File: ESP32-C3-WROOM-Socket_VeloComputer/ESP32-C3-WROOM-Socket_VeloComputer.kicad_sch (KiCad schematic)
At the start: 29 parts, among them J1 I2C, J3 Reed_Speed_Socket, J4 USB-C_Receptacle_Data_16P_GCT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, J5 Conn_01x02_Socket, J6 Speed_01x02_Pin, J7 Cadense_01x02_Pin, SW1 SW_Push_SMD_6x3.5, SW2 ENABLE, SW3 SW_Reed_Speed, SW4 SW_Reed_Cadence, U1 ESP32-C3-WROOM-02-N4, U2 AMS1117-3V3, U3 74LS14

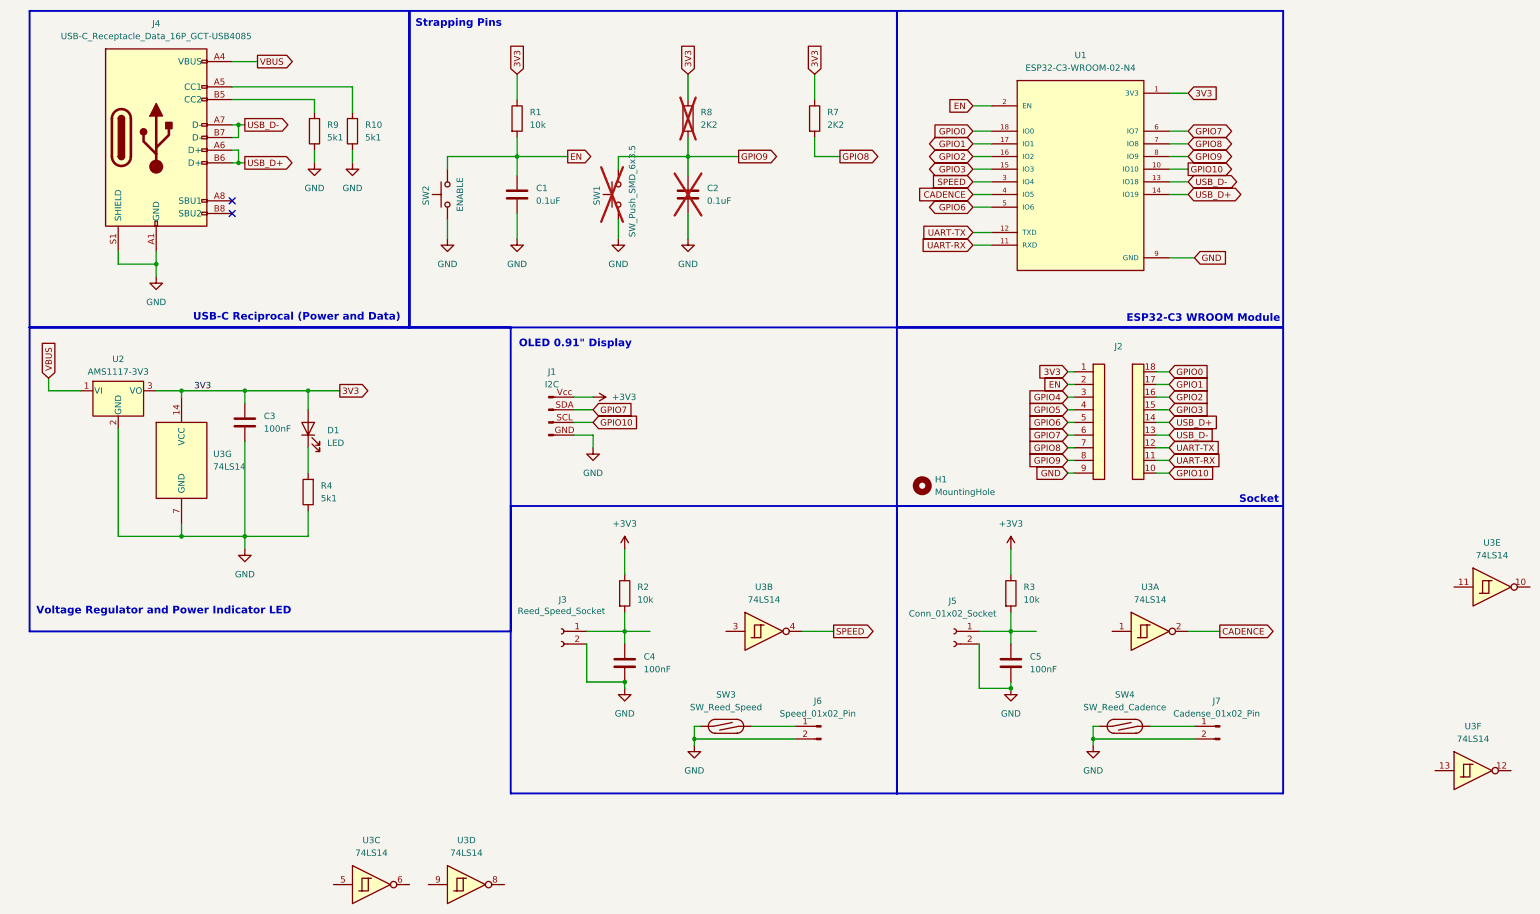
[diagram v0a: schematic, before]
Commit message: velocomputer
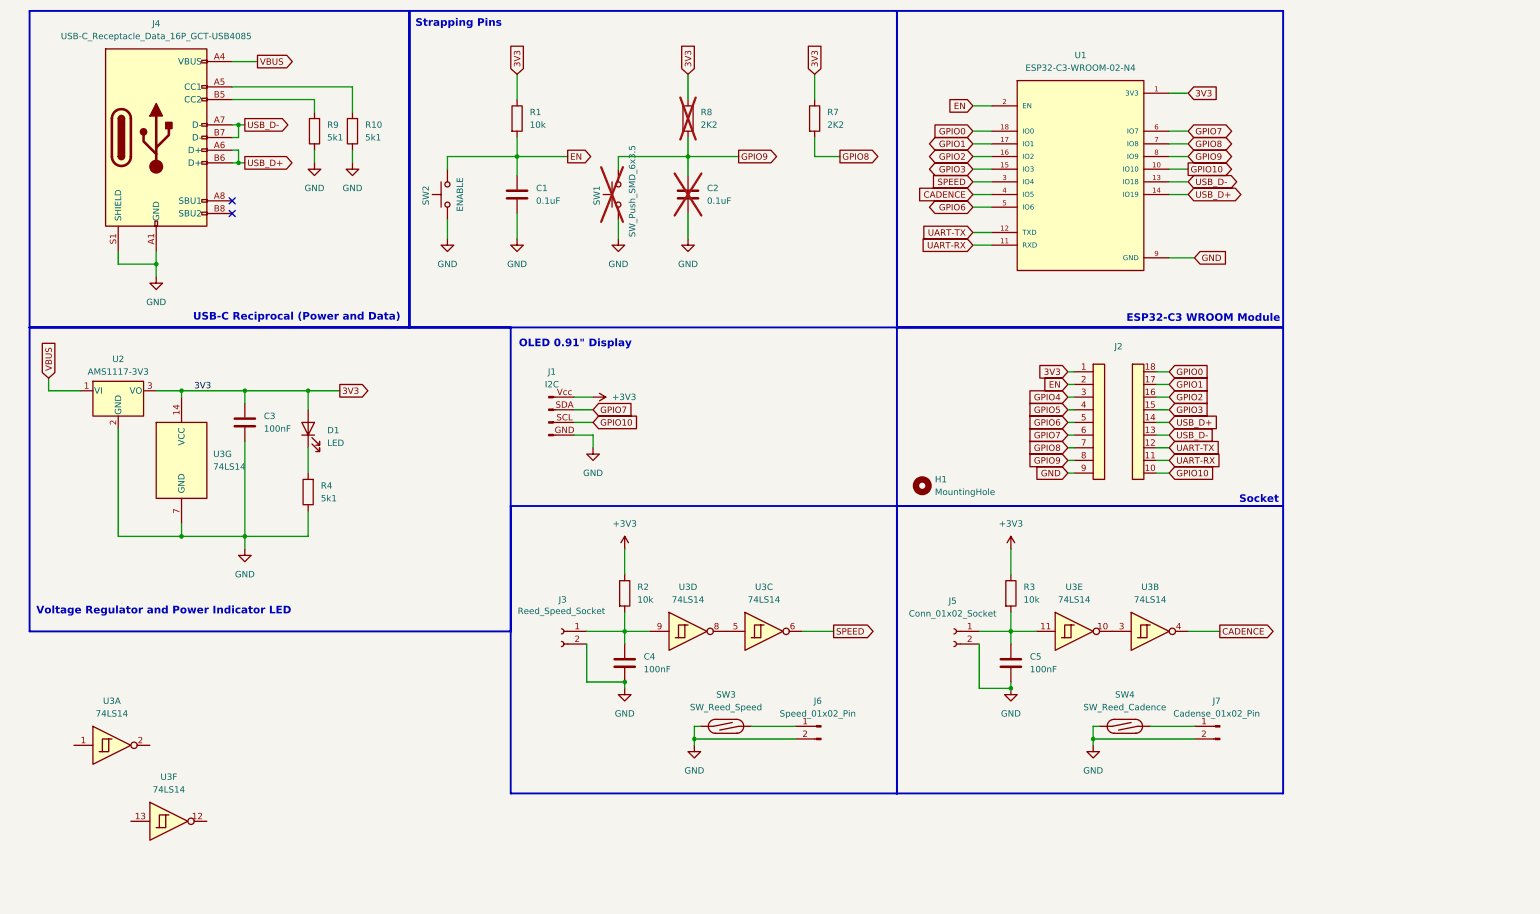
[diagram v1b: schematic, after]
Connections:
- net CADENCE: now also U3.4; no longer U3.2
- net SPEED: now also U3.6; no longer U3.4
- net at U3.5: now also U3.8
- net at U3.9: now also C4.1, J3.1 (Pin_1), R2.2
- net at C5.1, J5.1 (Pin_1), R3.2: now also U3.11
- net at U3.10: now also U3.3
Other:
- moved on the sheet: U3C, U3D, U3E

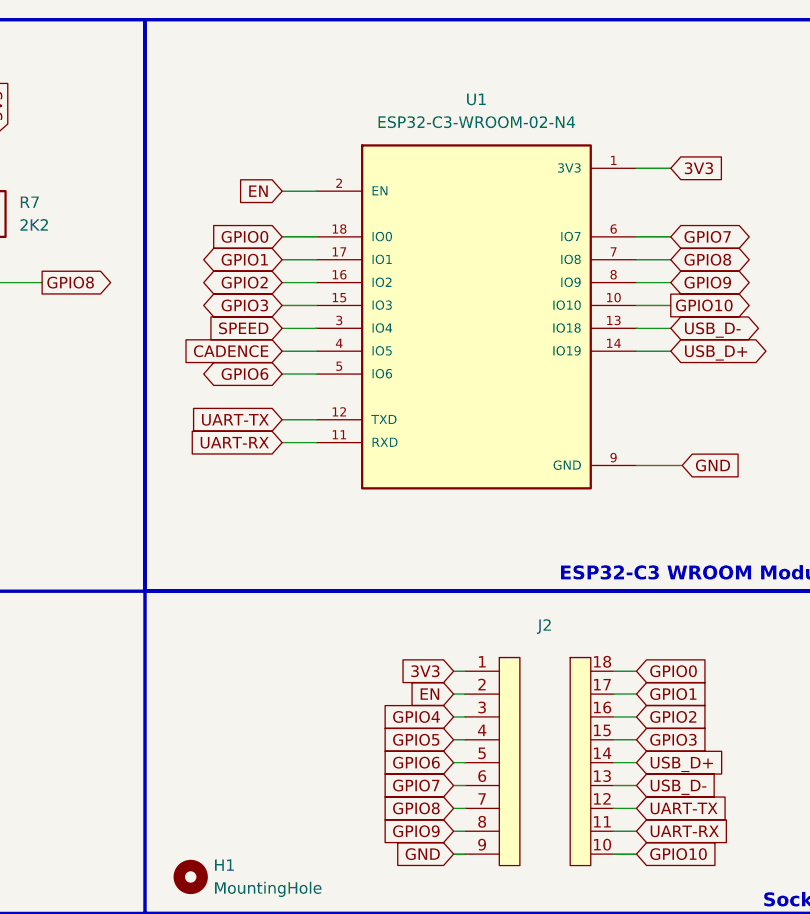
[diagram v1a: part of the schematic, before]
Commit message: velocomputer
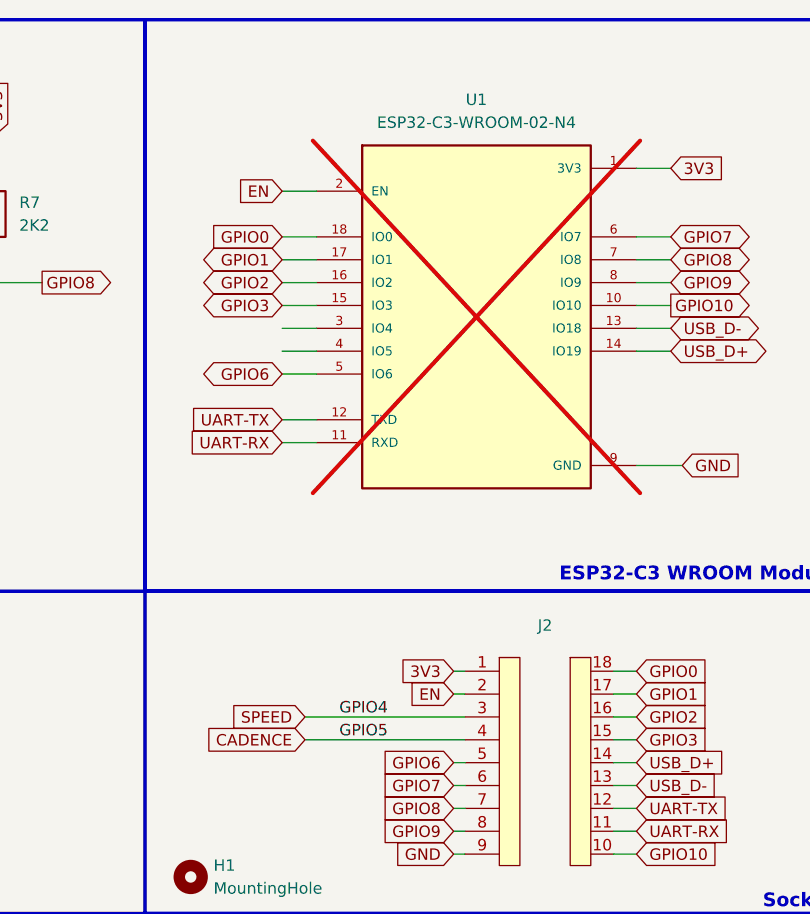
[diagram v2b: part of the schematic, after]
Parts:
- J2: now in the parts list
- U1: now not fitted; now left out of the parts list
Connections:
- net GPIO4 is gone; now on net SPEED: J2.3
- net GPIO5 is gone; now on net CADENCE: J2.4
- net CADENCE: no longer U1.4 (IO5)
- net SPEED: no longer U1.3 (IO4)
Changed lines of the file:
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@@
 	(wire
 		(pts
-			(xy 222.25 91.44) (xy 223.52 91.44)
+			(xy 205.74 91.44) (xy 223.52 91.44)
 		)
 		(stroke
@@
 	(wire
 		(pts
-			(xy 222.25 93.98) (xy 223.52 93.98)
+			(xy 205.74 93.98) (xy 223.52 93.98)
 		)
 		(stroke
@@
 		)
 	)
+	(label "GPIO4"
+		(at 209.55 91.44 0)
+		(effects
+			(font
+				(size 1.27 1.27)
+			)
+			(justify left bottom)
+		)
+	)
+	(label "GPIO5"
+		(at 209.55 93.98 0)
+		(effects
+			(font
+				(size 1.27 1.27)
+			)
+			(justify left bottom)
+		)
+	)
 	(label "3V3"
 		(at 46.99 90.17 0)
@@
 		)
 	)
-	(global_label "SPEED"
-		(shape input)
-		(at 203.2 48.26 180)
-		(fields_autoplaced yes)
-		(effects
-			(font
-				(size 1.27 1.27)
-			)
-			(justify right)
-		)
-		(property "Intersheetrefs" "${INTERSHEET_REFS}"
-			(at 194.1673 48.26 0)
-			(effects
-				(font
-					(size 1.27 1.27)
-				)
-				(justify right)
-				(hide yes)
-			)
-		)
-	)
 	(global_label "CADENCE"
 		(shape output)
@@
 		)
 	)
-	(global_label "GPIO5"
+	(global_label "UART-RX"
 		(shape input)
-		(at 222.25 93.98 180)
+		(at 203.2 60.96 180)
 		(fields_autoplaced yes)
 		(effects
@@
 		)
 		(property "Intersheetrefs" "${INTERSHEET_REFS}"
-			(at 213.58 93.98 0)
+			(at 191.5062 60.96 0)
 			(effects
 				(font
@@
 		)
 	)
-	(global_label "UART-RX"
+	(global_label "SPEED"
 		(shape input)
-		(at 203.2 60.96 180)
+		(at 205.74 91.44 180)
 		(fields_autoplaced yes)
 		(effects
@@
 		)
 		(property "Intersheetrefs" "${INTERSHEET_REFS}"
-			(at 191.5062 60.96 0)
+			(at 196.7073 91.44 0)
 			(effects
 				(font
@@
 		)
 	)
-	(global_label "CADENCE"
-		(shape input)
-		(at 203.2 50.8 180)
-		(fields_autoplaced yes)
-		(effects
-			(font
-				(size 1.27 1.27)
-			)
-			(justify right)
-		)
-		(property "Intersheetrefs" "${INTERSHEET_REFS}"
-			(at 191.6877 50.8 0)
-			(effects
-				(font
-					(size 1.27 1.27)
-				)
-				(justify right)
-				(hide yes)
-			)
-		)
-	)
 	(global_label "USB_D-"
 		(shape bidirectional)
@@
 		)
 	)
+	(global_label "CADENCE"
+		(shape input)
+		(at 205.74 93.98 180)
+		(fields_autoplaced yes)
+		(effects
+			(font
+				(size 1.27 1.27)
+			)
+			(justify right)
+		)
+		(property "Intersheetrefs" "${INTERSHEET_REFS}"
+			(at 194.2277 93.98 0)
+			(effects
+				(font
+					(size 1.27 1.27)
+				)
+				(justify right)
+				(hide yes)
+			)
+		)
+	)
 	(global_label "3V3"
 		(shape input)
@@
 		)
 	)
-	(global_label "GPIO4"
-		(shape input)
-		(at 222.25 91.44 180)
-		(fields_autoplaced yes)
-		(effects
-			(font
-				(size 1.27 1.27)
-			)
-			(justify right)
-		)
-		(property "Intersheetrefs" "${INTERSHEET_REFS}"
-			(at 213.58 91.44 0)
-			(effects
-				(font
-					(size 1.27 1.27)
-				)
-				(justify right)
-				(hide yes)
-			)
-		)
-	)
 	(global_label "GND"
 		(shape input)
@@
 		(unit 1)
 		(exclude_from_sim no)
-		(in_bom no)
-		(on_board no)
+		(in_bom yes)
+		(on_board yes)
 		(dnp no)
 		(fields_autoplaced yes)
@@
 		(unit 1)
 		(exclude_from_sim no)
-		(in_bom yes)
-		(on_board yes)
-		(dnp no)
+		(in_bom no)
+		(on_board no)
+		(dnp yes)
 		(fields_autoplaced yes)
 		(property "Reference" "U1"
